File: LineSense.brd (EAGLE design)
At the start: 100 x 45 mm, 45 parts, among them IC1 NJM2904M-TE1, IC2 NE555D, J1 1744426-4, Q1 SFH_3410-1_2-Z, Q2 2SC2712-GR,LF, Q3 2SC2712-GR,LF, Q5 2SC2712-GR,LF, Q6 2SC2712-GR,LF

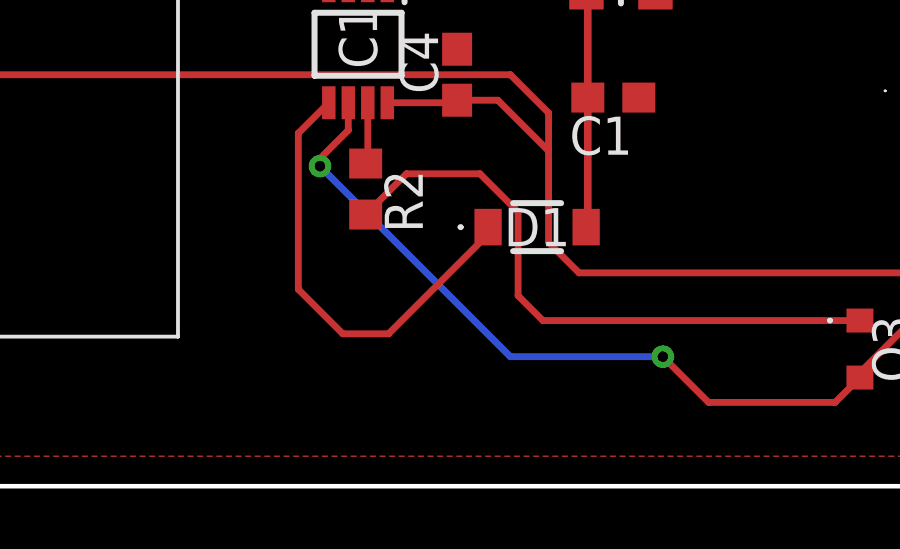
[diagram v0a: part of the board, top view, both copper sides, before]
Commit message: Revert "v1.2"
This reverts commit 20100e136a2bdf049fa62e188f43b768e8603774.
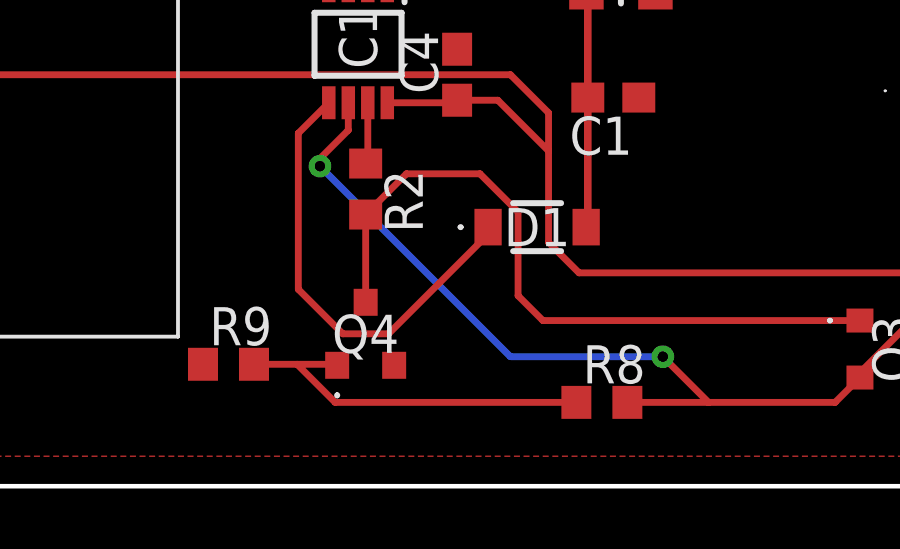
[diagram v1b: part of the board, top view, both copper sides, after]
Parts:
- added Q4: 2SC2712-GR,LF, SamacSys_Parts:SSM3J334RLF
- added R8: 3.6k, rcl:R0603
- added R9: 620, rcl:R0603
- R1: value 560k -> 500k
- R13: value 4.7k -> 7.5k
- R2, R7: value 0 -> 10k
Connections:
- net +5V renamed +12V
- new net N$10: Q4.1, R8.1, R9.2
- net GND: now also Q4.2, R9.1
- net N$8: now also Q4.3
- net SIG_OUT: now also R8.2
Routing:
- net N$10: track 0.00 -> 12.6 mm
- net N$8: track 20.7 -> 23.6 mm
- net SIG_OUT: track 60.4 -> 63.2 mm
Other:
- board text removed: "LineSense v1.1"
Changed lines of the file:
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@@
 <vertex x="82" y="20"/>
 </polygon>
-<text x="20" y="40" size="1.778" layer="26" rot="MR0">LineSense v1.1</text>
 </plain>
 <attributes>
@@
 <attribute name="VALUE" x="54.864" y="4.572" size="1.27" layer="27" rot="R270" align="center"/>
 </element>
+<element name="Q4" library="SamacSys_Parts" package="SSM3J334RLF" value="2SC2712-GR,LF" x="37.338" y="5.08" smashed="yes">
+<attribute name="ARROW_PART_NUMBER" value="2SC2712-GR,LF" x="88.138" y="-24.13" size="1.778" layer="27" display="off"/>
+<attribute name="ARROW_PRICE-STOCK" value="https://www.arrow.com/en/products/2sc2712-grlf/toshiba?region=nac" x="88.138" y="-24.13" size="1.778" layer="27" display="off"/>
+<attribute name="DESCRIPTION" value="Bipolar Transistors - BJT Transistor Lo Freq 0.15A 50V" x="88.138" y="-24.13" size="1.778" layer="27" display="off"/>
+<attribute name="HEIGHT" value="0.88mm" x="88.138" y="-24.13" size="1.778" layer="27" display="off"/>
+<attribute name="MANUFACTURER_NAME" value="Toshiba" x="88.138" y="-24.13" size="1.778" layer="27" display="off"/>
+<attribute name="MANUFACTURER_PART_NUMBER" value="2SC2712-GR,LF" x="88.138" y="-24.13" size="1.778" layer="27" display="off"/>
+<attribute name="MOUSER_PART_NUMBER" value="757-2SC2712-GRLF" x="88.138" y="-24.13" size="1.778" layer="27" display="off"/>
+<attribute name="MOUSER_PRICE-STOCK" value="https://www.mouser.co.uk/ProductDetail/Toshiba/2SC2712-GRLF?qs=OLJpxlzHOSROHaH%2Fh9sb9g%3D%3D" x="88.138" y="-24.13" size="1.778" layer="27" display="off"/>
+<attribute name="NAME" x="37.338" y="5.08" size="1.27" layer="25" align="center"/>
+<attribute name="VALUE" x="37.338" y="5.08" size="1.27" layer="27" align="center"/>
+</element>
 <element name="Q5" library="SamacSys_Parts" package="SSM3J334RLF" value="2SC2712-GR,LF" x="70.941" y="8.002" smashed="yes" rot="R270">
 <attribute name="ARROW_PART_NUMBER" value="2SC2712-GR,LF" x="35.381" y="-12.318" size="1.778" layer="27" rot="R270" display="off"/>
@@
 <attribute name="VALUE" x="87.836" y="9.306" size="1.27" layer="27" align="center"/>
 </element>
-<element name="R1" library="rcl" library_urn="urn:adsk.eagle:library:334" package="R0603" package3d_urn="urn:adsk.eagle:package:23555/3" value="560k" x="23.2918" y="27.432" smashed="yes" rot="R270">
+<element name="R1" library="rcl" library_urn="urn:adsk.eagle:library:334" package="R0603" package3d_urn="urn:adsk.eagle:package:23555/3" value="500k" x="23.2918" y="27.432" smashed="yes" rot="R270">
 <attribute name="NAME" x="23.9268" y="28.067" size="1.27" layer="25" rot="R270"/>
 <attribute name="POPULARITY" value="70" x="-17.3482" y="-3.048" size="1.778" layer="27" rot="R270" display="off"/>
@@
 <attribute name="VALUE" x="90.691" y="3.11" size="1.27" layer="27" rot="R90"/>
 </element>
-<element name="R13" library="rcl" library_urn="urn:adsk.eagle:library:334" package="R0603" package3d_urn="urn:adsk.eagle:package:23555/3" value="4.7k" x="71.986" y="14.402" smashed="yes" rot="R90">
+<element name="R13" library="rcl" library_urn="urn:adsk.eagle:library:334" package="R0603" package3d_urn="urn:adsk.eagle:package:23555/3" value="7.5k" x="71.986" y="14.402" smashed="yes" rot="R90">
 <attribute name="NAME" x="71.351" y="13.767" size="1.27" layer="25" rot="R90"/>
 <attribute name="POPULARITY" value="70" x="112.626" y="71.552" size="1.778" layer="27" rot="R90" display="off"/>
@@
 <attribute name="VALUE" x="80.137" y="21.463" size="1.27" layer="27" rot="R90"/>
 </element>
-<element name="R2" library="rcl" library_urn="urn:adsk.eagle:library:334" package="R0603" package3d_urn="urn:adsk.eagle:package:23555/3" value="0" x="37.338" y="9.906" smashed="yes" rot="R270">
+<element name="R2" library="rcl" library_urn="urn:adsk.eagle:library:334" package="R0603" package3d_urn="urn:adsk.eagle:package:23555/3" value="10k" x="37.338" y="9.906" smashed="yes" rot="R270">
 <attribute name="NAME" x="37.973" y="10.541" size="1.27" layer="25" rot="R270"/>
 <attribute name="POPULARITY" value="70" x="-13.462" y="-6.604" size="1.778" layer="27" rot="R270" display="off"/>
@@
 <attribute name="VALUE" x="37.973" y="25.019" size="1.27" layer="27"/>
 </element>
-<element name="R7" library="rcl" library_urn="urn:adsk.eagle:library:334" package="R0603" package3d_urn="urn:adsk.eagle:package:23555/3" value="0" x="39.37" y="19.812" smashed="yes" rot="R180">
+<element name="R7" library="rcl" library_urn="urn:adsk.eagle:library:334" package="R0603" package3d_urn="urn:adsk.eagle:package:23555/3" value="10k" x="39.37" y="19.812" smashed="yes" rot="R180">
 <attribute name="NAME" x="40.005" y="19.177" size="1.27" layer="25" rot="R180"/>
 <attribute name="POPULARITY" value="70" x="17.78" y="70.612" size="1.778" layer="27" rot="R180" display="off"/>
 <attribute name="SPICEPREFIX" value="R" x="17.78" y="70.612" size="1.778" layer="27" rot="R180" display="off"/>
 <attribute name="VALUE" x="40.005" y="21.717" size="1.27" layer="27" rot="R180"/>
+</element>
+<element name="R8" library="rcl" library_urn="urn:adsk.eagle:library:334" package="R0603" package3d_urn="urn:adsk.eagle:package:23555/3" value="3.6k" x="45.212" y="2.794" smashed="yes">
+<attribute name="NAME" x="44.577" y="3.429" size="1.27" layer="25"/>
+<attribute name="POPULARITY" value="70" x="97.282" y="-37.846" size="1.778" layer="27" display="off"/>
+<attribute name="SPICEPREFIX" value="R" x="97.282" y="-37.846" size="1.778" layer="27" display="off"/>
+<attribute name="VALUE" x="44.577" y="0.889" size="1.27" layer="27"/>
+</element>
+<element name="R9" library="rcl" library_urn="urn:adsk.eagle:library:334" package="R0603" package3d_urn="urn:adsk.eagle:package:23555/3" value="620" x="32.766" y="4.064" smashed="yes">
+<attribute name="NAME" x="32.131" y="4.699" size="1.27" layer="25"/>
+<attribute name="POPULARITY" value="70" x="89.916" y="-41.656" size="1.778" layer="27" display="off"/>
+<attribute name="SPICEPREFIX" value="R" x="89.916" y="-41.656" size="1.778" layer="27" display="off"/>
+<attribute name="VALUE" x="32.131" y="2.159" size="1.27" layer="27"/>
 </element>
 <element name="TP1" library="testpad" library_urn="urn:adsk.eagle:library:385" package="B1,27" package3d_urn="urn:adsk.eagle:package:27944/2" value="TPB1,27" x="76.93" y="15.24" smashed="yes">
@@
 <contactref element="R2" pad="2"/>
 <contactref element="Q3" pad="1"/>
+<contactref element="Q4" pad="3"/>
+<wire x1="37.338" y1="9.056" x2="37.338" y2="6.13" width="0.2286" layer="1"/>
 <wire x1="37.338" y1="9.056" x2="38.696" y2="10.414" width="0.2286" layer="1"/>
 <wire x1="38.696" y1="10.414" x2="41.148" y2="10.414" width="0.2286" layer="1"/>
@@
 <signal name="SIG_OUT">
 <contactref element="Q3" pad="2"/>
+<contactref element="R8" pad="2"/>
 <contactref element="IC1" pad="6"/>
 <contactref element="J1" pad="2"/>
 <contactref element="TP5" pad="TP"/>
+<wire x1="46.062" y1="2.794" x2="48.768" y2="2.794" width="0.2286" layer="1"/>
 <wire x1="48.768" y1="2.794" x2="52.986" y2="2.794" width="0.2286" layer="1"/>
 <wire x1="52.986" y1="2.794" x2="53.814" y2="3.622" width="0.2286" layer="1"/>
@@
 <wire x1="53.814" y1="3.78683125" x2="53.814" y2="3.622" width="0.2286" layer="1"/>
 </signal>
+<signal name="N$10">
+<contactref element="R8" pad="1"/>
+<contactref element="R9" pad="2"/>
+<contactref element="Q4" pad="1"/>
+<wire x1="33.616" y1="4.064" x2="35.052" y2="4.064" width="0.2286" layer="1"/>
+<wire x1="35.052" y1="4.064" x2="36.354" y2="4.064" width="0.2286" layer="1"/>
+<wire x1="36.354" y1="4.064" x2="36.388" y2="4.03" width="0.2286" layer="1"/>
+<wire x1="35.052" y1="4.064" x2="36.322" y2="2.794" width="0.2286" layer="1"/>
+<wire x1="36.322" y1="2.794" x2="44.362" y2="2.794" width="0.2286" layer="1"/>
+</signal>
 <signal name="N$14">
 <contactref element="D1" pad="2"/>
@@
 <contactref element="IC1" pad="4"/>
 <contactref element="C4" pad="2"/>
+<contactref element="Q4" pad="2"/>
+<contactref element="R9" pad="1"/>
 <contactref element="R11" pad="1"/>
 <contactref element="J1" pad="4"/>
@@
 </polygon>
 </signal>
-<signal name="+5V">
+<signal name="+12V">
 <contactref element="IC1" pad="8"/>
 <contactref element="C4" pad="1"/>

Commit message: v1.2
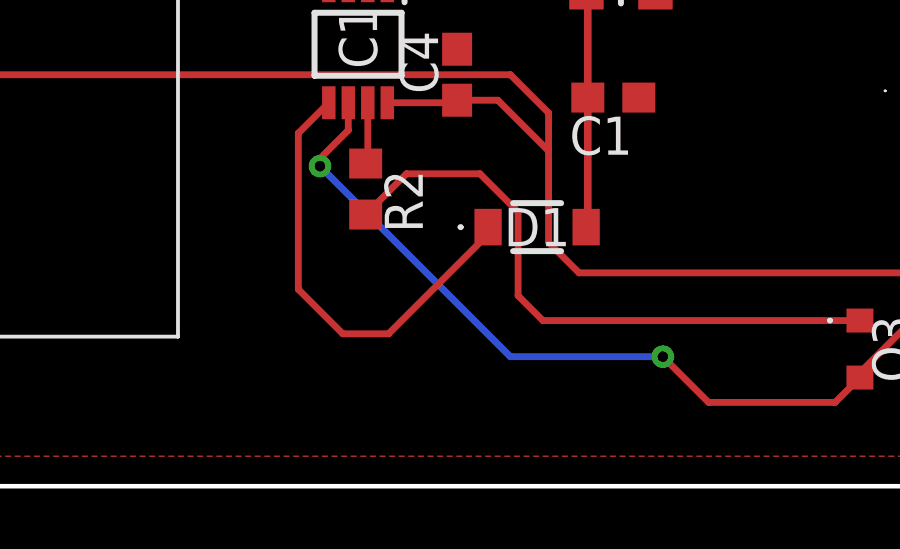
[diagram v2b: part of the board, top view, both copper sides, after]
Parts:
- removed Q4: 2SC2712-GR,LF, SamacSys_Parts:SSM3J334RLF
- removed R8: 3.6k, rcl:R0603
- removed R9: 620, rcl:R0603
- R1: value 500k -> 560k
- R13: value 7.5k -> 4.7k
- R2, R7: value 10k -> 0
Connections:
- net +12V renamed +5V
- removed net N$10: Q4.1, R8.1, R9.2
- net GND: no longer Q4.2, R9.1
- net N$8: no longer Q4.3
- net SIG_OUT: no longer R8.2
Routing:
- net N$10: track 12.6 -> 0.00 mm
- net N$8: track 23.6 -> 20.7 mm
- net SIG_OUT: track 63.2 -> 60.4 mm
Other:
- board text added: "LineSense v1.1"
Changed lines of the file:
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@@
 <vertex x="82" y="20"/>
 </polygon>
+<text x="20" y="40" size="1.778" layer="26" rot="MR0">LineSense v1.1</text>
 </plain>
 <attributes>
@@
 <attribute name="VALUE" x="54.864" y="4.572" size="1.27" layer="27" rot="R270" align="center"/>
 </element>
-<element name="Q4" library="SamacSys_Parts" package="SSM3J334RLF" value="2SC2712-GR,LF" x="37.338" y="5.08" smashed="yes">
-<attribute name="ARROW_PART_NUMBER" value="2SC2712-GR,LF" x="88.138" y="-24.13" size="1.778" layer="27" display="off"/>
-<attribute name="ARROW_PRICE-STOCK" value="https://www.arrow.com/en/products/2sc2712-grlf/toshiba?region=nac" x="88.138" y="-24.13" size="1.778" layer="27" display="off"/>
-<attribute name="DESCRIPTION" value="Bipolar Transistors - BJT Transistor Lo Freq 0.15A 50V" x="88.138" y="-24.13" size="1.778" layer="27" display="off"/>
-<attribute name="HEIGHT" value="0.88mm" x="88.138" y="-24.13" size="1.778" layer="27" display="off"/>
-<attribute name="MANUFACTURER_NAME" value="Toshiba" x="88.138" y="-24.13" size="1.778" layer="27" display="off"/>
-<attribute name="MANUFACTURER_PART_NUMBER" value="2SC2712-GR,LF" x="88.138" y="-24.13" size="1.778" layer="27" display="off"/>
-<attribute name="MOUSER_PART_NUMBER" value="757-2SC2712-GRLF" x="88.138" y="-24.13" size="1.778" layer="27" display="off"/>
-<attribute name="MOUSER_PRICE-STOCK" value="https://www.mouser.co.uk/ProductDetail/Toshiba/2SC2712-GRLF?qs=OLJpxlzHOSROHaH%2Fh9sb9g%3D%3D" x="88.138" y="-24.13" size="1.778" layer="27" display="off"/>
-<attribute name="NAME" x="37.338" y="5.08" size="1.27" layer="25" align="center"/>
-<attribute name="VALUE" x="37.338" y="5.08" size="1.27" layer="27" align="center"/>
-</element>
 <element name="Q5" library="SamacSys_Parts" package="SSM3J334RLF" value="2SC2712-GR,LF" x="70.941" y="8.002" smashed="yes" rot="R270">
 <attribute name="ARROW_PART_NUMBER" value="2SC2712-GR,LF" x="35.381" y="-12.318" size="1.778" layer="27" rot="R270" display="off"/>
@@
 <attribute name="VALUE" x="87.836" y="9.306" size="1.27" layer="27" align="center"/>
 </element>
-<element name="R1" library="rcl" library_urn="urn:adsk.eagle:library:334" package="R0603" package3d_urn="urn:adsk.eagle:package:23555/3" value="500k" x="23.2918" y="27.432" smashed="yes" rot="R270">
+<element name="R1" library="rcl" library_urn="urn:adsk.eagle:library:334" package="R0603" package3d_urn="urn:adsk.eagle:package:23555/3" value="560k" x="23.2918" y="27.432" smashed="yes" rot="R270">
 <attribute name="NAME" x="23.9268" y="28.067" size="1.27" layer="25" rot="R270"/>
 <attribute name="POPULARITY" value="70" x="-17.3482" y="-3.048" size="1.778" layer="27" rot="R270" display="off"/>
@@
 <attribute name="VALUE" x="90.691" y="3.11" size="1.27" layer="27" rot="R90"/>
 </element>
-<element name="R13" library="rcl" library_urn="urn:adsk.eagle:library:334" package="R0603" package3d_urn="urn:adsk.eagle:package:23555/3" value="7.5k" x="71.986" y="14.402" smashed="yes" rot="R90">
+<element name="R13" library="rcl" library_urn="urn:adsk.eagle:library:334" package="R0603" package3d_urn="urn:adsk.eagle:package:23555/3" value="4.7k" x="71.986" y="14.402" smashed="yes" rot="R90">
 <attribute name="NAME" x="71.351" y="13.767" size="1.27" layer="25" rot="R90"/>
 <attribute name="POPULARITY" value="70" x="112.626" y="71.552" size="1.778" layer="27" rot="R90" display="off"/>
@@
 <attribute name="VALUE" x="80.137" y="21.463" size="1.27" layer="27" rot="R90"/>
 </element>
-<element name="R2" library="rcl" library_urn="urn:adsk.eagle:library:334" package="R0603" package3d_urn="urn:adsk.eagle:package:23555/3" value="10k" x="37.338" y="9.906" smashed="yes" rot="R270">
+<element name="R2" library="rcl" library_urn="urn:adsk.eagle:library:334" package="R0603" package3d_urn="urn:adsk.eagle:package:23555/3" value="0" x="37.338" y="9.906" smashed="yes" rot="R270">
 <attribute name="NAME" x="37.973" y="10.541" size="1.27" layer="25" rot="R270"/>
 <attribute name="POPULARITY" value="70" x="-13.462" y="-6.604" size="1.778" layer="27" rot="R270" display="off"/>
@@
 <attribute name="VALUE" x="37.973" y="25.019" size="1.27" layer="27"/>
 </element>
-<element name="R7" library="rcl" library_urn="urn:adsk.eagle:library:334" package="R0603" package3d_urn="urn:adsk.eagle:package:23555/3" value="10k" x="39.37" y="19.812" smashed="yes" rot="R180">
+<element name="R7" library="rcl" library_urn="urn:adsk.eagle:library:334" package="R0603" package3d_urn="urn:adsk.eagle:package:23555/3" value="0" x="39.37" y="19.812" smashed="yes" rot="R180">
 <attribute name="NAME" x="40.005" y="19.177" size="1.27" layer="25" rot="R180"/>
 <attribute name="POPULARITY" value="70" x="17.78" y="70.612" size="1.778" layer="27" rot="R180" display="off"/>
 <attribute name="SPICEPREFIX" value="R" x="17.78" y="70.612" size="1.778" layer="27" rot="R180" display="off"/>
 <attribute name="VALUE" x="40.005" y="21.717" size="1.27" layer="27" rot="R180"/>
-</element>
-<element name="R8" library="rcl" library_urn="urn:adsk.eagle:library:334" package="R0603" package3d_urn="urn:adsk.eagle:package:23555/3" value="3.6k" x="45.212" y="2.794" smashed="yes">
-<attribute name="NAME" x="44.577" y="3.429" size="1.27" layer="25"/>
-<attribute name="POPULARITY" value="70" x="97.282" y="-37.846" size="1.778" layer="27" display="off"/>
-<attribute name="SPICEPREFIX" value="R" x="97.282" y="-37.846" size="1.778" layer="27" display="off"/>
-<attribute name="VALUE" x="44.577" y="0.889" size="1.27" layer="27"/>
-</element>
-<element name="R9" library="rcl" library_urn="urn:adsk.eagle:library:334" package="R0603" package3d_urn="urn:adsk.eagle:package:23555/3" value="620" x="32.766" y="4.064" smashed="yes">
-<attribute name="NAME" x="32.131" y="4.699" size="1.27" layer="25"/>
-<attribute name="POPULARITY" value="70" x="89.916" y="-41.656" size="1.778" layer="27" display="off"/>
-<attribute name="SPICEPREFIX" value="R" x="89.916" y="-41.656" size="1.778" layer="27" display="off"/>
-<attribute name="VALUE" x="32.131" y="2.159" size="1.27" layer="27"/>
 </element>
 <element name="TP1" library="testpad" library_urn="urn:adsk.eagle:library:385" package="B1,27" package3d_urn="urn:adsk.eagle:package:27944/2" value="TPB1,27" x="76.93" y="15.24" smashed="yes">
@@
 <contactref element="R2" pad="2"/>
 <contactref element="Q3" pad="1"/>
-<contactref element="Q4" pad="3"/>
-<wire x1="37.338" y1="9.056" x2="37.338" y2="6.13" width="0.2286" layer="1"/>
 <wire x1="37.338" y1="9.056" x2="38.696" y2="10.414" width="0.2286" layer="1"/>
 <wire x1="38.696" y1="10.414" x2="41.148" y2="10.414" width="0.2286" layer="1"/>
@@
 <signal name="SIG_OUT">
 <contactref element="Q3" pad="2"/>
-<contactref element="R8" pad="2"/>
 <contactref element="IC1" pad="6"/>
 <contactref element="J1" pad="2"/>
 <contactref element="TP5" pad="TP"/>
-<wire x1="46.062" y1="2.794" x2="48.768" y2="2.794" width="0.2286" layer="1"/>
 <wire x1="48.768" y1="2.794" x2="52.986" y2="2.794" width="0.2286" layer="1"/>
 <wire x1="52.986" y1="2.794" x2="53.814" y2="3.622" width="0.2286" layer="1"/>
@@
 <wire x1="53.814" y1="3.78683125" x2="53.814" y2="3.622" width="0.2286" layer="1"/>
 </signal>
-<signal name="N$10">
-<contactref element="R8" pad="1"/>
-<contactref element="R9" pad="2"/>
-<contactref element="Q4" pad="1"/>
-<wire x1="33.616" y1="4.064" x2="35.052" y2="4.064" width="0.2286" layer="1"/>
-<wire x1="35.052" y1="4.064" x2="36.354" y2="4.064" width="0.2286" layer="1"/>
-<wire x1="36.354" y1="4.064" x2="36.388" y2="4.03" width="0.2286" layer="1"/>
-<wire x1="35.052" y1="4.064" x2="36.322" y2="2.794" width="0.2286" layer="1"/>
-<wire x1="36.322" y1="2.794" x2="44.362" y2="2.794" width="0.2286" layer="1"/>
-</signal>
 <signal name="N$14">
 <contactref element="D1" pad="2"/>
@@
 <contactref element="IC1" pad="4"/>
 <contactref element="C4" pad="2"/>
-<contactref element="Q4" pad="2"/>
-<contactref element="R9" pad="1"/>
 <contactref element="R11" pad="1"/>
 <contactref element="J1" pad="4"/>
@@
 </polygon>
 </signal>
-<signal name="+12V">
+<signal name="+5V">
 <contactref element="IC1" pad="8"/>
 <contactref element="C4" pad="1"/>
